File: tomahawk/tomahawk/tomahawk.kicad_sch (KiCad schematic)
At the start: 80 parts, among them SW1 SW_Push, SW10 SW_Push, SW11 SW_Push, SW12 SW_Push, SW13 SW_Push, SW14 SW_Push, SW15 SW_Push, SW16 SW_Push, SW17 SW_Push, SW18 SW_Push, SW19 SW_Push, SW2 SW_Push, SW20 SW_Push, SW21 SW_Push, SW22 SW_Push, SW23 SW_Push, SW24 SW_Push, SW25 SW_Push, SW26 SW_Push, SW27 SW_Push, SW28 SW_Push, SW29 SW_Push, SW3 SW_Push, SW30 SW_Push, SW31 SW_Push, SW32 SW_Push, SW33 SW_Push, SW34 SW_Push, SW35 SW_Push, SW36 SW_Push, SW37 SW_Push, SW38 SW_Push, SW39 SW_Push, SW4 SW_Push, SW5 SW_Push, SW6 SW_Push, SW7 SW_Push, SW8 SW_Push, SW9 SW_Push, U2 nice_nano

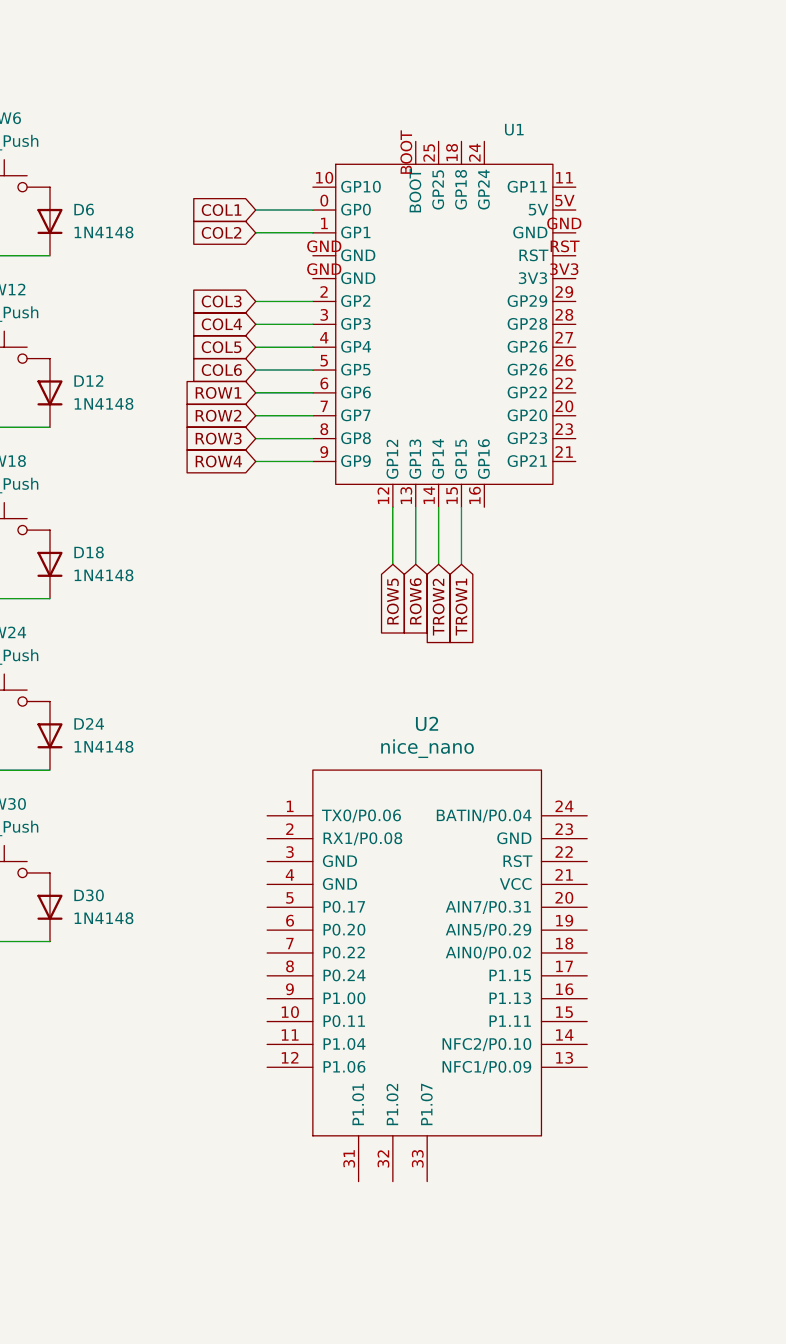
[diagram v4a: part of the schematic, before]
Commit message: wip
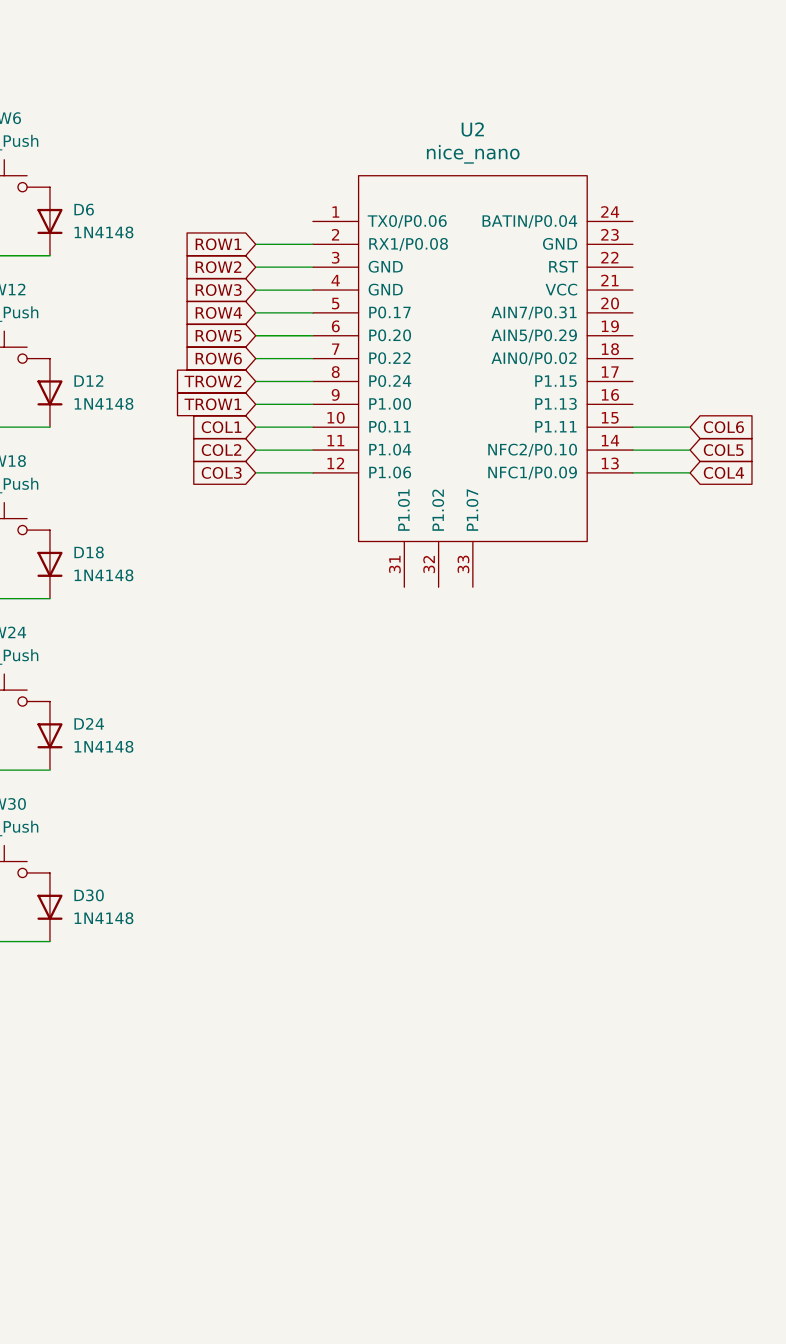
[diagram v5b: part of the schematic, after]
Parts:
- removed U1: ~, ProMicro RP2040:pro_micro_rp2040, symbol ProMicro_RP2040:pro_micro_rp2040
- D1, D10, D11, D12, D13, D14, D15, D16, D17, D18, D19, D2, D20, D21, D22, D23, D24, D25, D26, D27, D28, D29, D3, D30, D31, D32, D33, D34, D35, D36, D37, D38, D39, D4, D5, D6, D7, D8, D9: footprint Diode_THT:D_DO-35_SOD27_P7.62mm_Horizontal -> Diode_SMD:D_SOD-123
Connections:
- net COL1: now also U2.10 (P0.11)
- net COL2: now also U2.11 (P1.04)
- net COL3: now also U2.12 (P1.06)
- net COL4: now also U2.13 (NFC1/P0.09)
- net COL5: now also U2.14 (NFC2/P0.10)
- net COL6: now also U2.15 (P1.11)
- net ROW1: now also U2.2 (RX1/P0.08)
- net ROW2: now also U2.3 (GND)
- net ROW3: now also U2.4 (GND)
- net ROW4: now also U2.5 (P0.17)
- net ROW5: now also U2.6 (P0.20)
- net ROW6: now also U2.7 (P0.22)
- net TROW1: now also U2.9 (P1.00)
- net TROW2: now also U2.8 (P0.24)
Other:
- moved on the sheet: U2
